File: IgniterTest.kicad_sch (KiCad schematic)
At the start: 16 parts

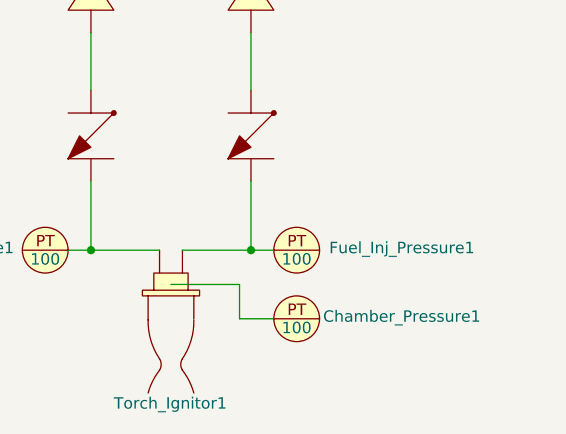
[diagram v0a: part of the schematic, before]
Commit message: ho tin leung
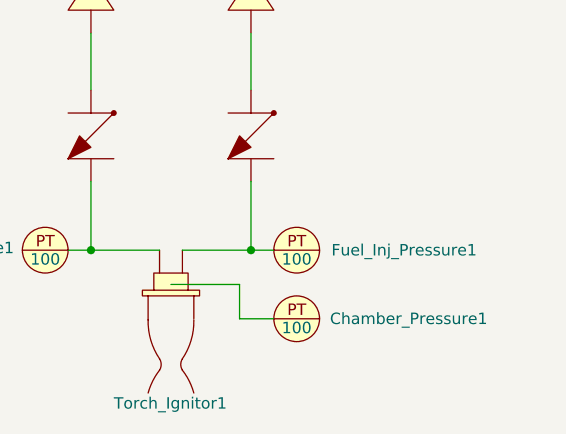
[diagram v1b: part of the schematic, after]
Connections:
- net at Fuel_Main_Servo1.: now also Check_Valve6.; no longer Fuel_Tank1.
- net at N2_Line_Vent_Manual1.: now also Fuel_Press1., N2_Reg1.
- net at N2_Bottle1.: now also N2_Reg1.
- net at N2O_Bottle1.: now also Ox_Main_Servo1.
- net at Ox_Main_Servo1.: now also Check_Valve5.; no longer N2O_Bottle1.
- new net: Check_Valve6., Fuel_Inj_Pressure1., Torch_Ignitor1.
- new net: Check_Valve5., Ox_Inj_Pressure1., Torch_Ignitor1.
- new net: Fuel_Main_Servo1., Fuel_Tank1.
- now unconnected: Fuel_Inj_Pressure1., Ox_Inj_Pressure1.
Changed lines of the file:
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@@
+				)
+			)
+			(project "IgniterTest"
+				(path "/1fe58bd7-d6db-4cdb-9816-3cf1e5c4b0ec"
+					(reference "Torch_Ignitor")
+					(unit 1)
 				)
 			)
@@
 		(dnp no)
 		(property "Reference" "Chamber_Pressure1"
-			(at 151.384 157.226 0)
+			(at 152.146 157.48 0)
 			(effects
 				(font
@@
 				(path "/045f1f05-3134-4b6d-91b6-463031104f1e/6a55bbd5-ed21-4b79-a194-d378f68dea1b"
 					(reference "Chamber_Pressure1")
+					(unit 1)
+				)
+			)
+			(project "IgniterTest"
+				(path "/1fe58bd7-d6db-4cdb-9816-3cf1e5c4b0ec"
+					(reference "Chamber_Pressure")
 					(unit 1)
 				)
@@
 				)
 			)
+			(project "IgniterTest"
+				(path "/1fe58bd7-d6db-4cdb-9816-3cf1e5c4b0ec"
+					(reference "Fuel_Main_Servo")
+					(unit 1)
+				)
+			)
 		)
 	)
@@
 				(path "/045f1f05-3134-4b6d-91b6-463031104f1e/6a55bbd5-ed21-4b79-a194-d378f68dea1b"
 					(reference "N2_Line_Vent_Manual1")
+					(unit 1)
+				)
+			)
+			(project "IgniterTest"
+				(path "/1fe58bd7-d6db-4cdb-9816-3cf1e5c4b0ec"
+					(reference "N2_Line_Vent_Manual")
 					(unit 1)
 				)
@@
 				)
 			)
+			(project "IgniterTest"
+				(path "/1fe58bd7-d6db-4cdb-9816-3cf1e5c4b0ec"
+					(reference "N2_Bottle")
+					(unit 1)
+				)
+			)
 		)
 	)
@@
 				)
 			)
+			(project "IgniterTest"
+				(path "/1fe58bd7-d6db-4cdb-9816-3cf1e5c4b0ec"
+					(reference "Fuel_Tank")
+					(unit 1)
+				)
+			)
 		)
 	)
@@
 		(dnp no)
 		(property "Reference" "Fuel_Inj_Pressure1"
-			(at 151.384 149.606 0)
+			(at 151.638 149.86 0)
 			(effects
 				(font
@@
 				(path "/045f1f05-3134-4b6d-91b6-463031104f1e/6a55bbd5-ed21-4b79-a194-d378f68dea1b"
 					(reference "Fuel_Inj_Pressure1")
+					(unit 1)
+				)
+			)
+			(project "IgniterTest"
+				(path "/1fe58bd7-d6db-4cdb-9816-3cf1e5c4b0ec"
+					(reference "Fuel_Inj_Pressure")
 					(unit 1)
 				)
@@
 				)
 			)
+			(project "IgniterTest"
+				(path "/1fe58bd7-d6db-4cdb-9816-3cf1e5c4b0ec"
+					(reference "Ox_Inj_Pressure")
+					(unit 1)
+				)
+			)
 		)
 	)
@@
 				)
 			)
-		)
-	)
-	(symbol
-		(lib_name "PID_symbols:Check_Valve")
+			(project "IgniterTest"
+				(path "/1fe58bd7-d6db-4cdb-9816-3cf1e5c4b0ec"
+					(reference "N2O_Bottle")
+					(unit 1)
+				)
+			)
+		)
+	)
+	(symbol
 		(lib_id "PID_symbols:Check_Valve")
 		(at 116.84 134.62 270)
@@
 				)
 			)
-		)
-	)
-	(symbol
-		(lib_name "PID_symbols:Check_Valve")
+			(project "IgniterTest"
+				(path "/1fe58bd7-d6db-4cdb-9816-3cf1e5c4b0ec"
+					(reference "Check_Valve?")
+					(unit 1)
+				)
+			)
+		)
+	)
+	(symbol
 		(lib_id "PID_symbols:Check_Valve")
 		(at 134.62 134.62 270)
@@
 				)
 			)
+			(project "IgniterTest"
+				(path "/1fe58bd7-d6db-4cdb-9816-3cf1e5c4b0ec"
+					(reference "Check_Valve?")
+					(unit 1)
+				)
+			)
 		)
 	)
@@
 				)
 			)
+			(project "IgniterTest"
+				(path "/1fe58bd7-d6db-4cdb-9816-3cf1e5c4b0ec"
+					(reference "Fuel_Tank_Pressure")
+					(unit 1)
+				)
+			)
 		)
 	)
@@
 				)
 			)
+			(project "IgniterTest"
+				(path "/1fe58bd7-d6db-4cdb-9816-3cf1e5c4b0ec"
+					(reference "Fuel_Vent_Servo")
+					(unit 1)
+				)
+			)
 		)
 	)
@@
 				)
 			)
+			(project "IgniterTest"
+				(path "/1fe58bd7-d6db-4cdb-9816-3cf1e5c4b0ec"
+					(reference "Fuel_Press")
+					(unit 1)
+				)
+			)
 		)
 	)
@@
 				(path "/045f1f05-3134-4b6d-91b6-463031104f1e/6a55bbd5-ed21-4b79-a194-d378f68dea1b"
 					(reference "N2_Reg1")
+					(unit 1)
+				)
+			)
+			(project "IgniterTest"
+				(path "/1fe58bd7-d6db-4cdb-9816-3cf1e5c4b0ec"
+					(reference "N2_Reg")
 					(unit 1)
 				)
@@
 				)
 			)
-		)
-	)
+			(project "IgniterTest"
+				(path "/1fe58bd7-d6db-4cdb-9816-3cf1e5c4b0ec"
+					(reference "Ox_Main_Servo")
+					(unit 1)
+				)
+			)
+		)
+	)
+	(sheet_instances
+		(path "/"
+			(page "1")
+		)
+	)
